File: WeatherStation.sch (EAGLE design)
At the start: 35 parts, among them J1 EDISON_CONNECTOR_FULLMOUNTING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, J2 EDISON_CONNECTOR_FULLHEADER, U1 MCP73831, U2 HTU21D, U3 MPL3115A2, U4 PCA9306

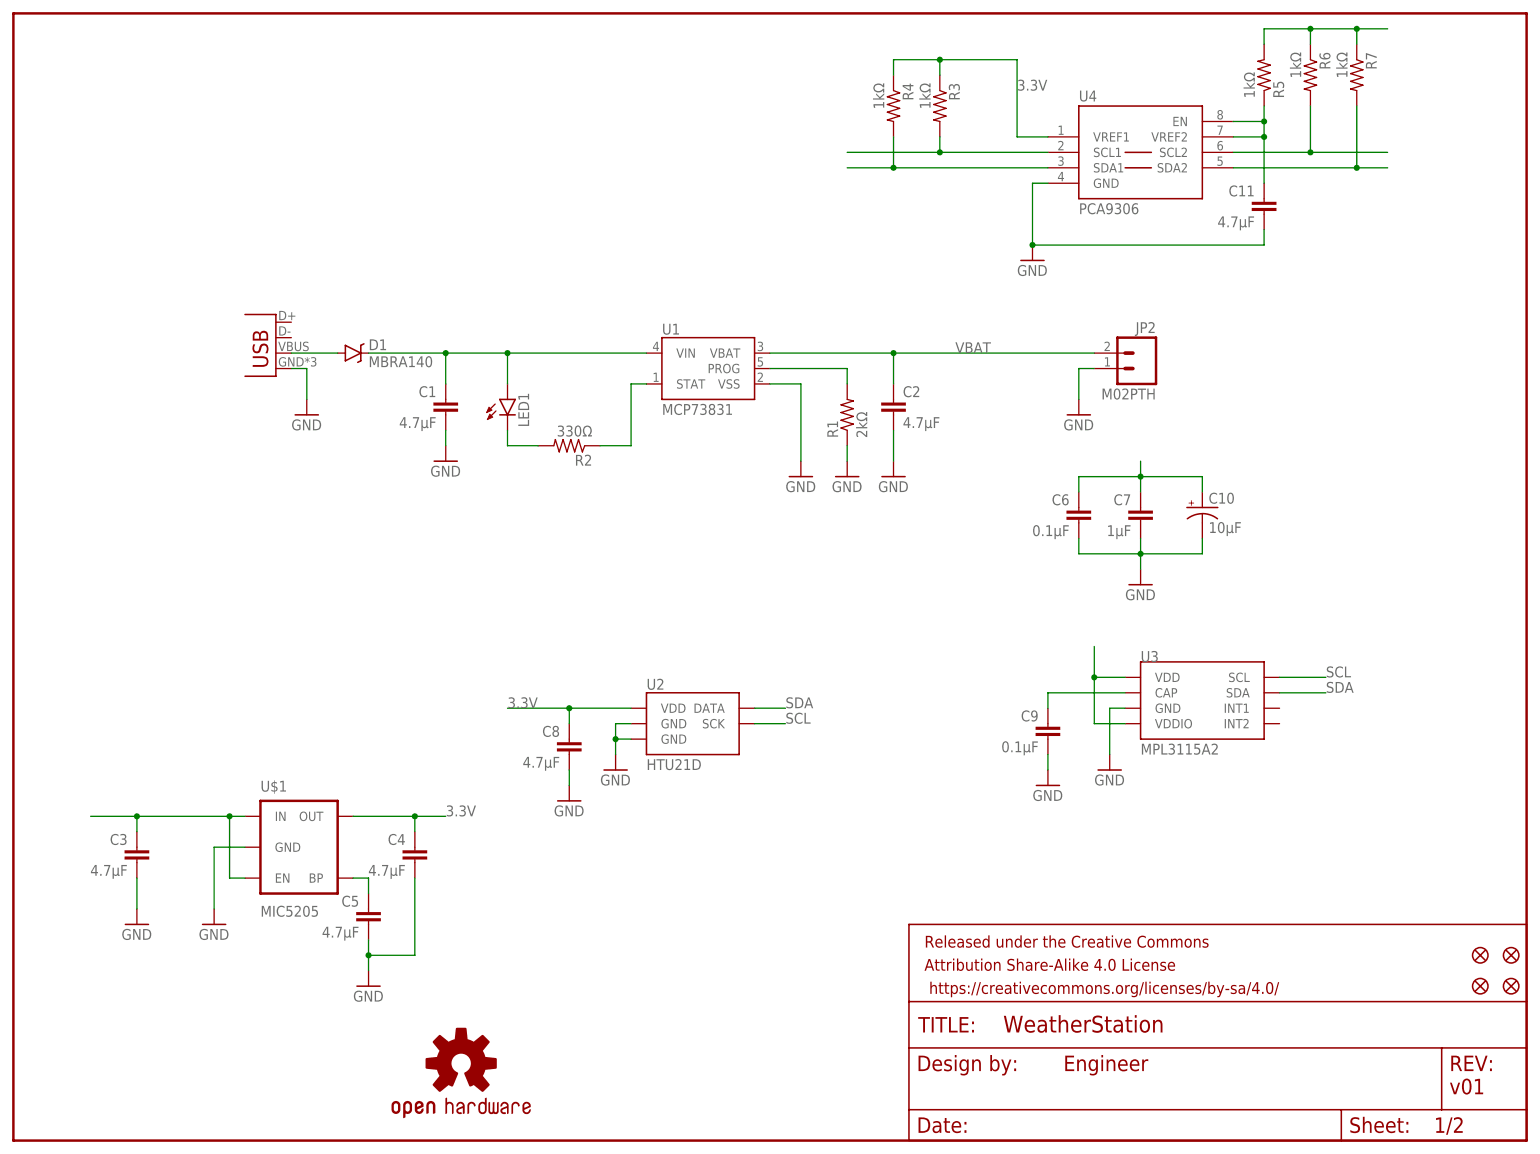
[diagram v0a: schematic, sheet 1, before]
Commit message: corrected values
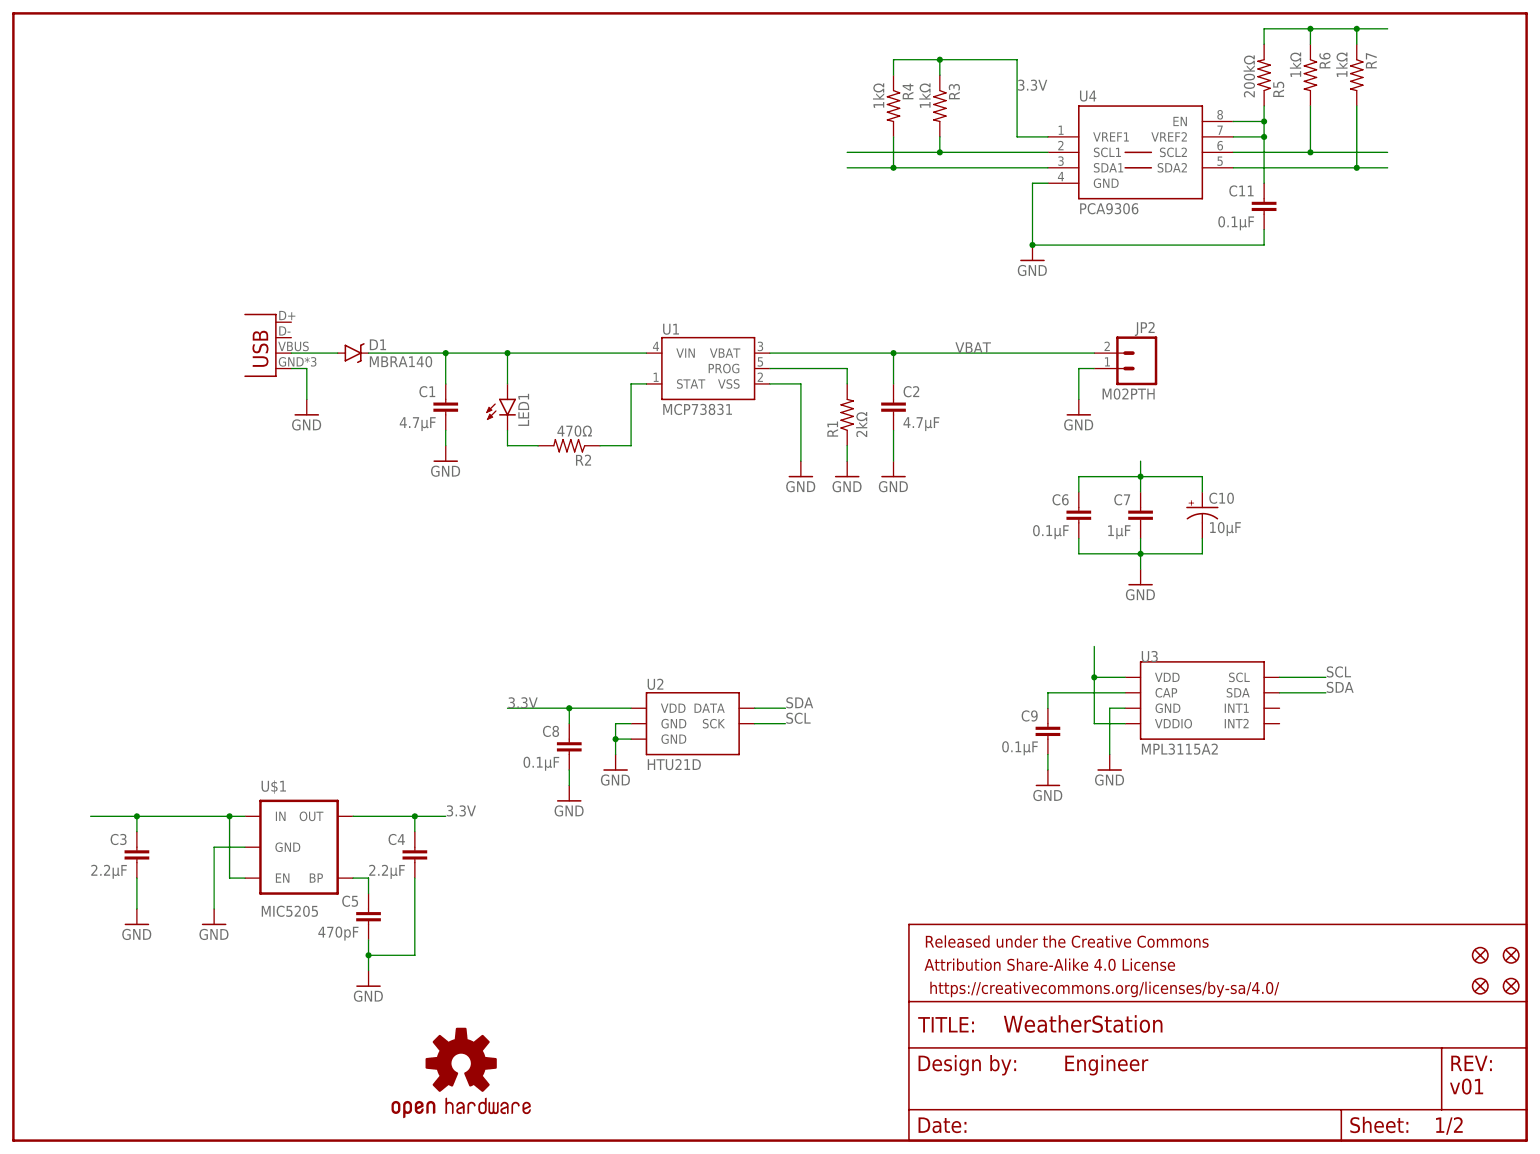
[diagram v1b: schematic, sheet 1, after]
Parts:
- C11, C8: value 4.7µF -> 0.1µF
- C3, C4: value 4.7µF -> 2.2µF
- C5: value 4.7µF -> 470pF
- R2: value 330Ω -> 470Ω
- R5: value 1kΩ -> 200kΩ
